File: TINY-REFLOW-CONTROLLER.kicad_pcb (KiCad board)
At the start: 2 copper layers, 40 x 51 mm, 51 parts, among them J1 TERMINAL-BLOCK-1x2, J2 TERMINAL-BLOCK-1x2, J3 MICRO-USB, J4 2.54mm 2x3, J5 2.54mm 1x6, M1 MOUNT_HOLE, M2 MOUNT_HOLE, M3 MOUNT_HOLE, M4 MOUNT_HOLE, M5 FIDUCIAL, M6 FIDUCIAL, Q1 2N3904, Q2 2N3904, SW1 IT-1109S, SW2 IT-1109S, SW3 TS-018, U1 ATTINY1634R-MU, U2 MCP1700T-3302E/MB, U3 MAX31856, U4 RT0802A

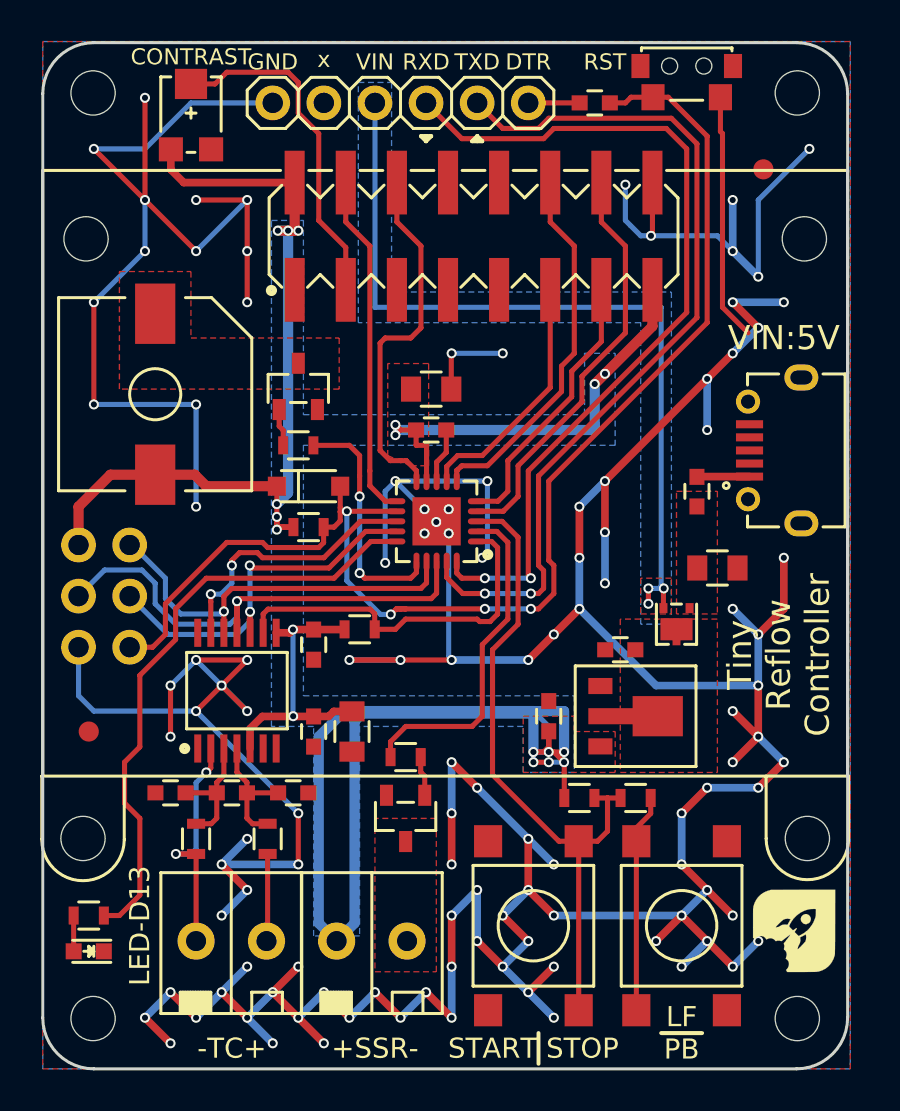
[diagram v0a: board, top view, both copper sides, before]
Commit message: Version 2.0
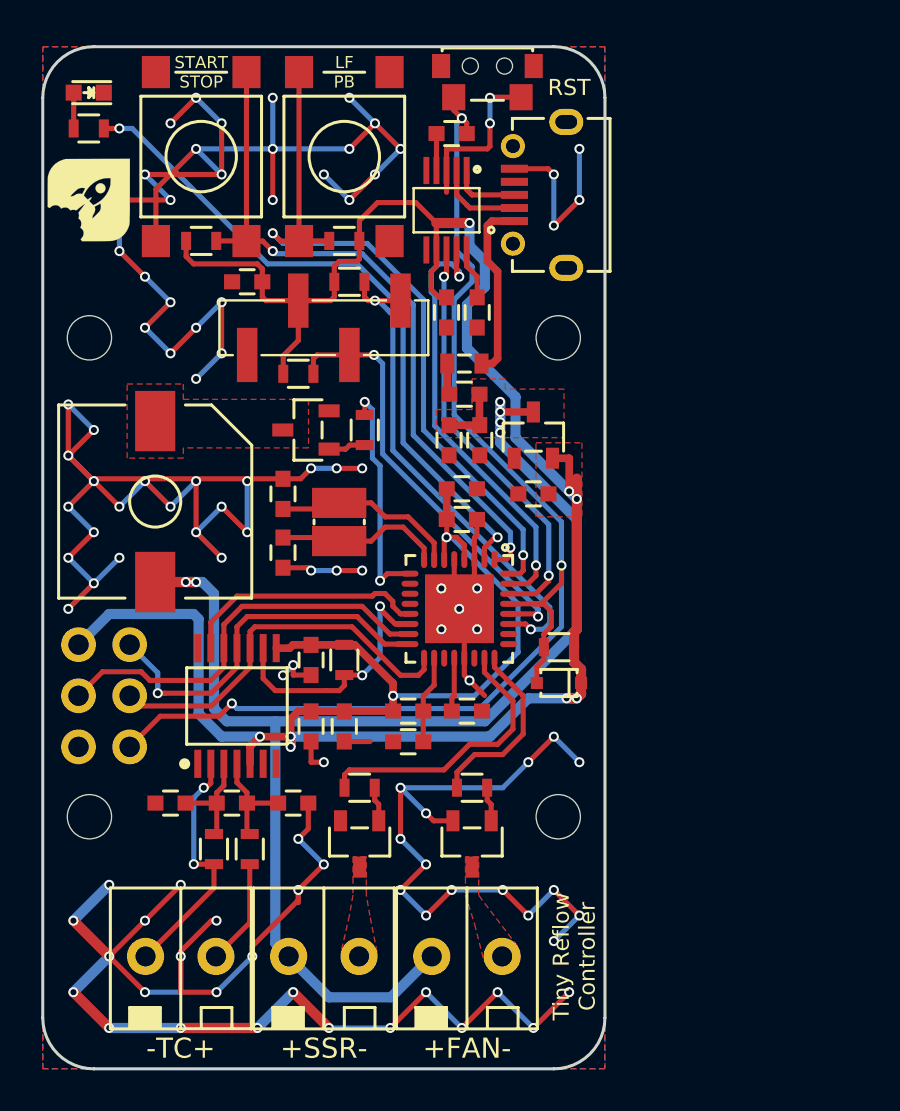
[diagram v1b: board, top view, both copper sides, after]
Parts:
- removed D2: PMEG3020CPA, RocketScreamKicadLibrary:SOT-1016
- removed M1, M2, M3, M4: MOUNT_HOLE, RocketScreamKicadLibrary:HOLE_NPTH_2.2MM
- removed M5, M6: FIDUCIAL, RocketScreamKicadLibrary:FIDUCIAL-1MM
- added C13: 100nF, RocketScreamKiCadLib:C_0603, F.Cu at (170.1, 62.4)
- added C14: 100nF, RocketScreamKiCadLib:C_0603, F.Cu at (171.6, 62.4)
- added C15: 10pF, RocketScreamKiCadLib:C_0603, F.Cu at (161.9, 71.4)
- added C16: 10pF, RocketScreamKiCadLib:C_0603, F.Cu at (161.9, 74.3)
- added C17: 100nF, RocketScreamKiCadLib:C_0603, F.Cu at (168.2, 83.7)
- added C18: 100nF, RocketScreamKiCadLib:C_0603, F.Cu at (171.1, 82.2)
- added C19: 100nF, RocketScreamKiCadLib:C_0603, F.Cu at (160.2, 60.9)
- added F1: FUSE, RocketScreamKiCadLib:MF-FSMF, F.Cu at (171.0, 64.9)
- added L2: LBMF1608T100K, RocketScreamKiCadLib:I_0603, F.Cu at (168.2, 82.2)
- added Q3: 2N3904, RocketScreamKiCadLib:SOT-23, F.Cu at (171.3, 88.8)
- added R11: 2K2, RocketScreamKiCadLib:R_0603, F.Cu at (165.2, 60.9)
- added R12: 53K6, RocketScreamKiCadLib:R_0603, F.Cu at (171.3, 86.0)
- added U5: OLED-SSD1306-128X64-I2C, RocketScreamKiCadLib:OLED-SSD1306-128X64-I2C, F.Cu at (164.0, 63.2)
- added Y1: NX3225GD, RocketScreamKiCadLib:NX3225GD, F.Cu at (164.7, 72.8)
- C1, C2, C3, C6, C7, C8, C9: footprint RocketScreamKicadLibrary:C_0603 -> RocketScreamKiCadLib:C_0603
- C10, C12: value 10uF 10V X5R -> 10uF 16V X5R; footprint RocketScreamKicadLibrary:C_0805 -> RocketScreamKiCadLib:C_0603
- C11: value 10uF 10V X5R -> 100nF; footprint RocketScreamKicadLibrary:C_0805 -> RocketScreamKiCadLib:C_0603
- C4: value 1uF 16V X7R -> 100nF; footprint RocketScreamKicadLibrary:C_0603 -> RocketScreamKiCadLib:C_0603
- C5: value 1uF 16V X7R -> 10uF 16V X5R; footprint RocketScreamKicadLibrary:C_0603 -> RocketScreamKiCadLib:C_0603
- D1: footprint RocketScreamKicadLibrary:LED_0603 -> RocketScreamKiCadLib:LED_0603
- D3: footprint RocketScreamKicadLibrary:SOD-123 -> RocketScreamKiCadLib:SOD-323
- J1, J2: footprint RocketScreamKicadLibrary:TB-1776275-2 -> RocketScreamKiCadLib:TB-1776275-2
- J3: footprint RocketScreamKicadLibrary:MICRO-USB -> RocketScreamKiCadLib:MICRO-USB
- J4: footprint RocketScreamKicadLibrary:HDR_2x3_Pitch2.54mm -> RocketScreamKiCadLib:HDR_2x3_Pitch2.54mm
- J5: value 2.54mm 1x6 -> TERMINAL-BLOCK-1x2; footprint RocketScreamKicadLibrary:HDR_1x6_Pitch2.54mm -> RocketScreamKiCadLib:TB-1776275-2
- L1: footprint RocketScreamKicadLibrary:I_0603 -> RocketScreamKiCadLib:I_0603
- LOGO1: footprint RocketScreamKicadLibrary:LOGO-ROCKET-SCREAM_Without_Text_XXXSmall -> RocketScreamKiCadLib:LOGO-ROCKET-SCREAM_Without_Text_XXXSmall
- LOGO2: footprint RocketScreamKicadLibrary:LOGO-KICAD -> RocketScreamKiCadLib:LOGO-KICAD_XSmall
- LOGO3: footprint RocketScreamKicadLibrary:LOGO-ROCKET-SCREAM_Vertical_Medium -> RocketScreamKiCadLib:LOGO-ROCKET-SCREAM_Vertical_Small
- LOGO4: footprint RocketScreamKicadLibrary:LOGO-OSHW_Small -> RocketScreamKiCadLib:LOGO-OSHW_Small
- LS1: footprint RocketScreamKicadLibrary:HYG9605B -> RocketScreamKiCadLib:HYG9605B
- Q1, Q2: footprint RocketScreamKicadLibrary:SOT-23 -> RocketScreamKiCadLib:SOT-23
- R1: value 35WR10KLFTR -> 2K2; footprint RocketScreamKicadLibrary:TC33X-x -> RocketScreamKiCadLib:R_0603
- R10, R2, R3, R4, R5, R6, R7, R8, R9: footprint RocketScreamKicadLibrary:R_0603 -> RocketScreamKiCadLib:R_0603
- SW1, SW2: footprint RocketScreamKicadLibrary:IT-1102W -> RocketScreamKiCadLib:IT-1102W
- SW3: footprint RocketScreamKicadLibrary:TS-018 -> RocketScreamKiCadLib:TS-018
- U1: value ATTINY1634R-MU -> ATMEGA328P-MU; footprint RocketScreamKicadLibrary:QFN-20_4x4mm -> RocketScreamKiCadLib:QFN-32_5x5mm_Pitch0.5mm
- U2: value MCP1700T-3302E/MB -> MCP1700T-3302E-TT; footprint RocketScreamKicadLibrary:SOT-89 -> RocketScreamKiCadLib:SOT-23
- U3: footprint RocketScreamKicadLibrary:TSSOP-14 -> RocketScreamKiCadLib:TSSOP-14
- U4: value RT0802A -> CH340E; footprint RocketScreamKicadLibrary:0802A-1-SMT -> RocketScreamKiCadLib:MSOP-10
- moved LOGO1 50.5 mm to (152.3, 56.8)
- moved D1 42.7 mm to (152.3, 51.5)
- moved J5 42.5 mm to (171.1, 94.4)
- moved SW2 41.7 mm to (165.0, 54.7)
- moved SW1 41.6 mm to (157.9, 54.7)
- moved R6 39.1 mm to (152.3, 53.3)
- moved R4 33.5 mm to (157.9, 58.9)
- moved R5 31.2 mm to (165.0, 58.9), turned to 180 degrees
- moved J3 17.3 mm to (174.9, 56.6)
- moved D3 15.8 mm to (175.7, 80.8), turned to 180 degrees
- moved U4 15.7 mm to (170.1, 57.3), turned to 180 degrees
- moved LOGO3 14.9 mm to (164.0, 79.9)
- moved U2 14.9 mm to (174.4, 68.5), turned to 0 degrees
- moved R1 14.0 mm to (162.7, 65.5)
- moved R9 13.8 mm to (175.7, 79.0), turned to 0 degrees
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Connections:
- C4 pad 1: VBUS -> 5V0
- J2 pad 1: 3V3 -> 5V0
- J3 pad 1: Net-(J3-Pad1) -> VUSB
- J4 pad 1: /D15 -> /D12
- J4 pad 3: /D12 -> /D13
- J4 pad 4: /D16 -> /D11
- J5 pad 1: Net-(C7-Pad1) -> 5V0
- J5 pad 2: /D0 -> Net-(J5-Pad2)
- L1 pad 1: Net-(J3-Pad1) -> Net-(F1-Pad2)
- LS1 pad 1: 3V3 -> 5V0
- R1 pad 2: Net-(R1-Pad2) -> /SCL
- R10 pad 2: /D2 -> /D10
- R4 pad 2: /D4 -> /D3
- R5 pad 1: /D4 -> 3V3
- R5 pad 2: Net-(R5-Pad2) -> /D2
- R6 pad 2: /D13 -> /D4
- R7 pad 1: /D14 -> /D5
- R8 pad 1: /D3 -> /A0
- SW1 pad 3: /D4 -> /D3
- SW1 pad 4: /D4 -> /D3
- SW2 pad 1: Net-(R5-Pad2) -> /D2
- SW2 pad 2: Net-(R5-Pad2) -> /D2
- U1 pad 1: /D2 -> /D3
- U1 pad 10: /D9 -> /D6
- U1 pad 11: /D10 -> /D7
- U1 pad 12: /RST -> /D8
- U1 pad 13: /D11 -> /D9
- U1 pad 14: /D12 -> /D10
- U1 pad 15: /D13 -> /D11
- U1 pad 16: /D14 -> /D12
- U1 pad 17: /D15 -> /D13
- U1 pad 18: /D16 -> Net-(C17-Pad1)
- U1 pad 19: /D0 -> /A6
- U1 pad 2: /D3 -> /D4
- U1 pad 20: /D1 -> AREF
- U1 pad 3: /D4 -> GND
- U1 pad 4: /D5 -> 3V3
- U1 pad 5: /D6 -> GND
- U1 pad 6: /D7 -> 3V3
- U1 pad 7: /D8 -> Net-(C15-Pad1)
- U1 pad 8: GND -> Net-(C16-Pad1)
- U1 pad 9: 3V3 -> /D5
- U2 pad 2: VBUS -> 3V3
- U2 pad 3: 3V3 -> 5V0
- U3 pad 10: /D12 -> /D13
- U3 pad 11: /D16 -> /D12
- U3 pad 12: /D15 -> /D11
- U3 pad 13: /D11 -> /D9
- U3 pad 9: /D2 -> /D10
- U4 pad 1: GND -> Net-(J3-Pad3)
- U4 pad 2: 3V3 -> Net-(J3-Pad2)
- U4 pad 3: Net-(R1-Pad2) -> GND
- U4 pad 4: /D10 -> Net-(C7-Pad1)
- U4 pad 5: GND -> Net-(U4-Pad5)
- U4 pad 6: /D9 -> Net-(U4-Pad6)
- U4 pad 7: Net-(U4-Pad7) -> 3V3
- U4 pad 8: Net-(U4-Pad8) -> /D0
- U4 pad 9: Net-(U4-Pad9) -> /D1
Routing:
- net GND: track 336.3 -> 253.9 mm, vias 116 -> 107
- net 5V0: track 0.00 -> 67.9 mm, vias 0 -> 6
- net VUSB: track 40.9 -> 9.16 mm, vias 3 -> 0
- net /D16: track 25.7 -> 0.00 mm, vias 1 -> 0
- net /SDA: track 0.00 -> 24.8 mm, vias 0 -> 2
- net /D0: track 43.7 -> 20.9 mm
- net 3V3: track 151.4 -> 129.5 mm, vias 18 -> 10
- net /SCL: track 0.00 -> 21.7 mm, vias 0 -> 2
- net /D1: track 43.3 -> 22.1 mm
- net /D15: track 20.0 -> 0.00 mm, vias 1 -> 0
- net /D7: track 18.5 -> 0.00 mm
- net /D2: track 18.4 -> 36.5 mm, vias 0 -> 2
- net /D3: track 16.8 -> 34.8 mm, vias 0 -> 2
- net Net-(R1-Pad2): track 17.1 -> 0.00 mm
- net /A0: track 0.00 -> 14.1 mm
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- added copper zone on F.Cu, net Net-(J5-Pad2)
- removed copper zone on B.Cu, net 3V3
- removed copper zone on F.Cu, net VBUS
- removed copper zone on B.Cu, net VUSB
- removed copper zone on F.Cu, net VUSB
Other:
- board size 40 x 51 mm -> 27.9 x 50.8 mm
- net class Default: clearance 0.203 -> 0.2032; trace_width 0.25 -> 0.254
- rule trace_clearance: 0.203 -> 0.2032
- board text added: "+FAN-"
- board text added: "2v00 12-2018"
- board text removed: "0v20 07-2017"
- board text removed: "CONTRAST"
- board text removed: "DTR"
- board text removed: "GND"
- board text removed: "LED-D13"
- board text removed: "RXD"
- board text removed: "TXD"
- board text removed: "VIN"
- board text removed: "VIN:5V"
- board text removed: "x"
